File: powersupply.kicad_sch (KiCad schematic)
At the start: 20 parts, among them U5 LMR14020, U6 AZ1117-3.3

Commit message: routed ad2s
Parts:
- C32: LCSC (none) -> C302008
- R27: LCSC (none) -> C25804
- R29: LCSC (none) -> C23231
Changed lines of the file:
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@@
+      (effects (font (size 1.27 1.27)) hide)
+    )
+    (property "LCSC" "C25804" (id 4) (at 127.635 96.52 0)
       (effects (font (size 1.27 1.27)) hide)
     )
@@
     )
     (property "Datasheet" "~" (id 3) (at 135.89 100.965 0)
+      (effects (font (size 1.27 1.27)) hide)
+    )
+    (property "LCSC" "C302008" (id 4) (at 135.89 100.965 0)
       (effects (font (size 1.27 1.27)) hide)
     )
@@
       (effects (font (size 1.27 1.27)) hide)
     )
+    (property "LCSC" "C23231" (id 4) (at 175.26 95.25 90)
+      (effects (font (size 1.27 1.27)) hide)
+    )

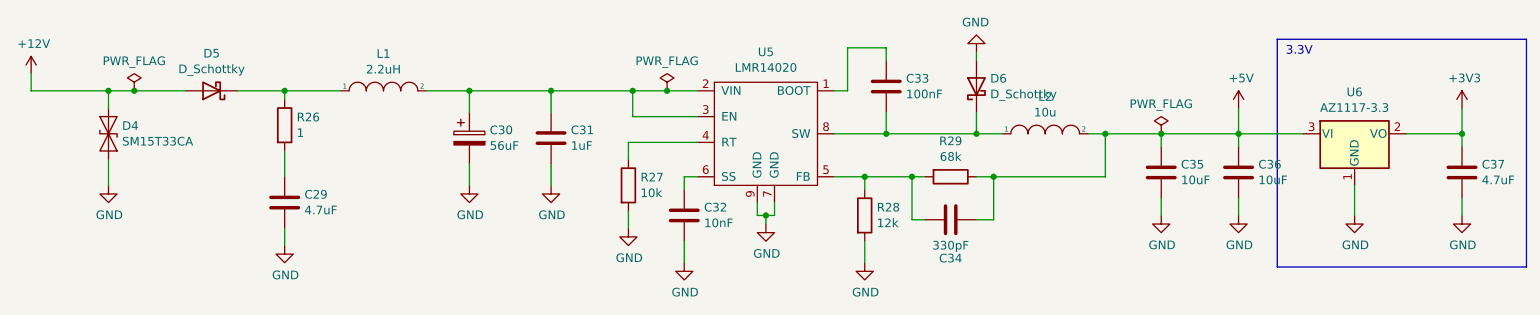
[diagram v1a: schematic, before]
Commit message: fixes for v5
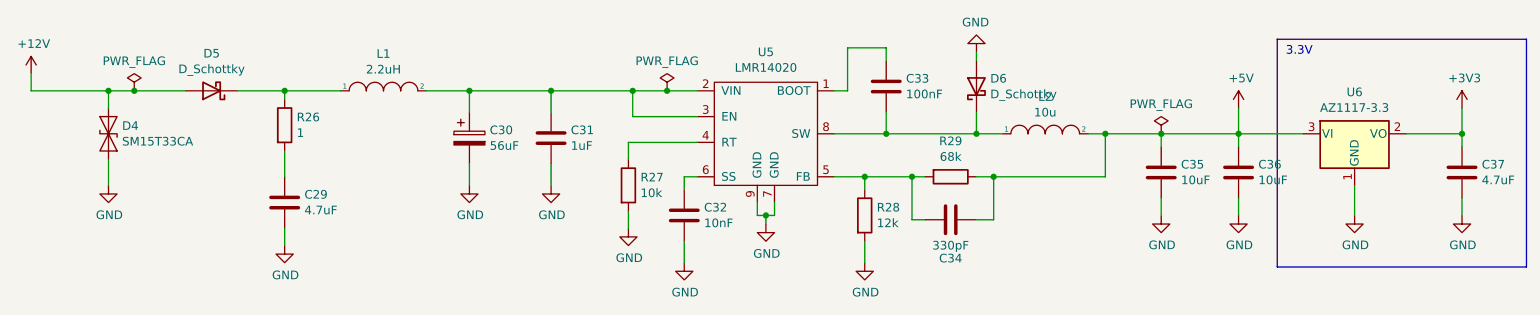
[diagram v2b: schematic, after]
